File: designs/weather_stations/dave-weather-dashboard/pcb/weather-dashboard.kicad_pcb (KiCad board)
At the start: 2 copper layers, 34.5 x 58 mm, 14 parts, among them J1 Conn_01x02_MountingPin, Q1 SL2301S, SW2 SW_Omron_B3FS, U1 WEMOS_S2_Mini, U3 MCP73831-2-OT, U4 U4

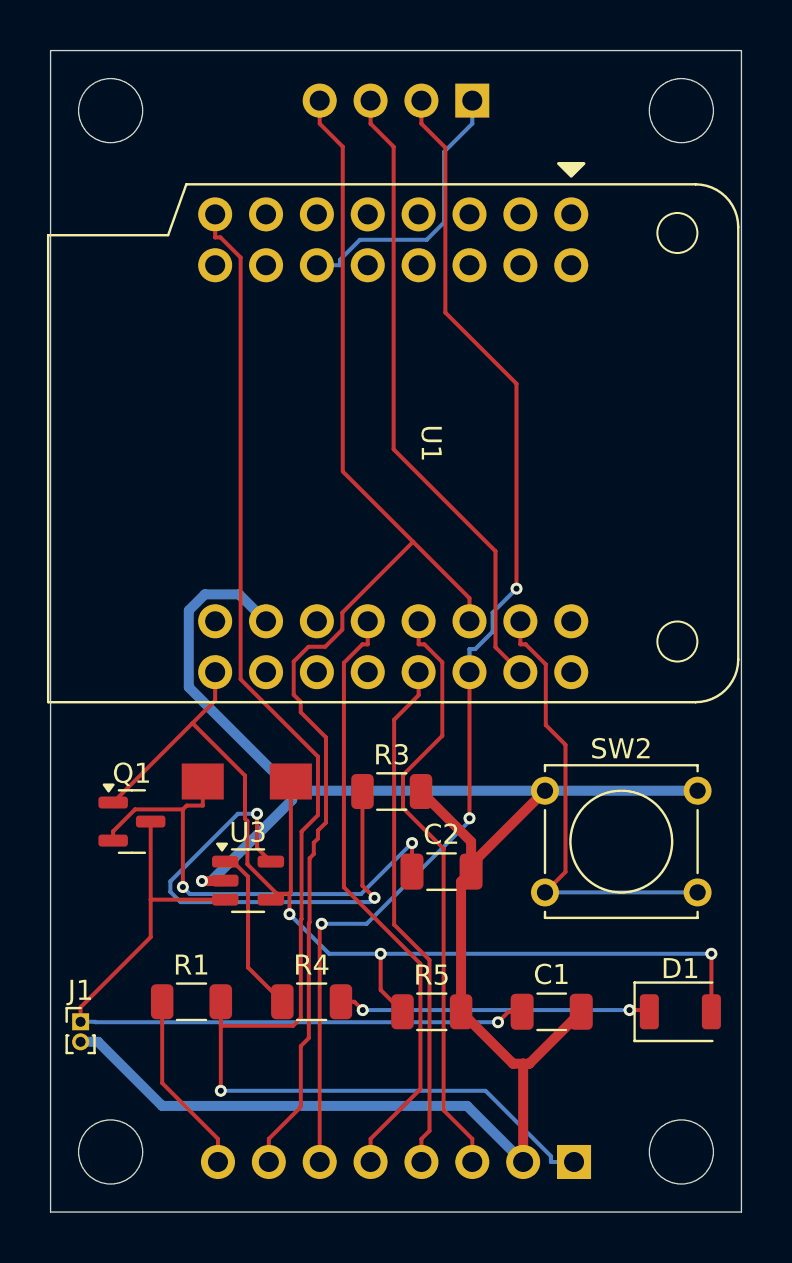
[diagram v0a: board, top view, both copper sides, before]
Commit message: done :)
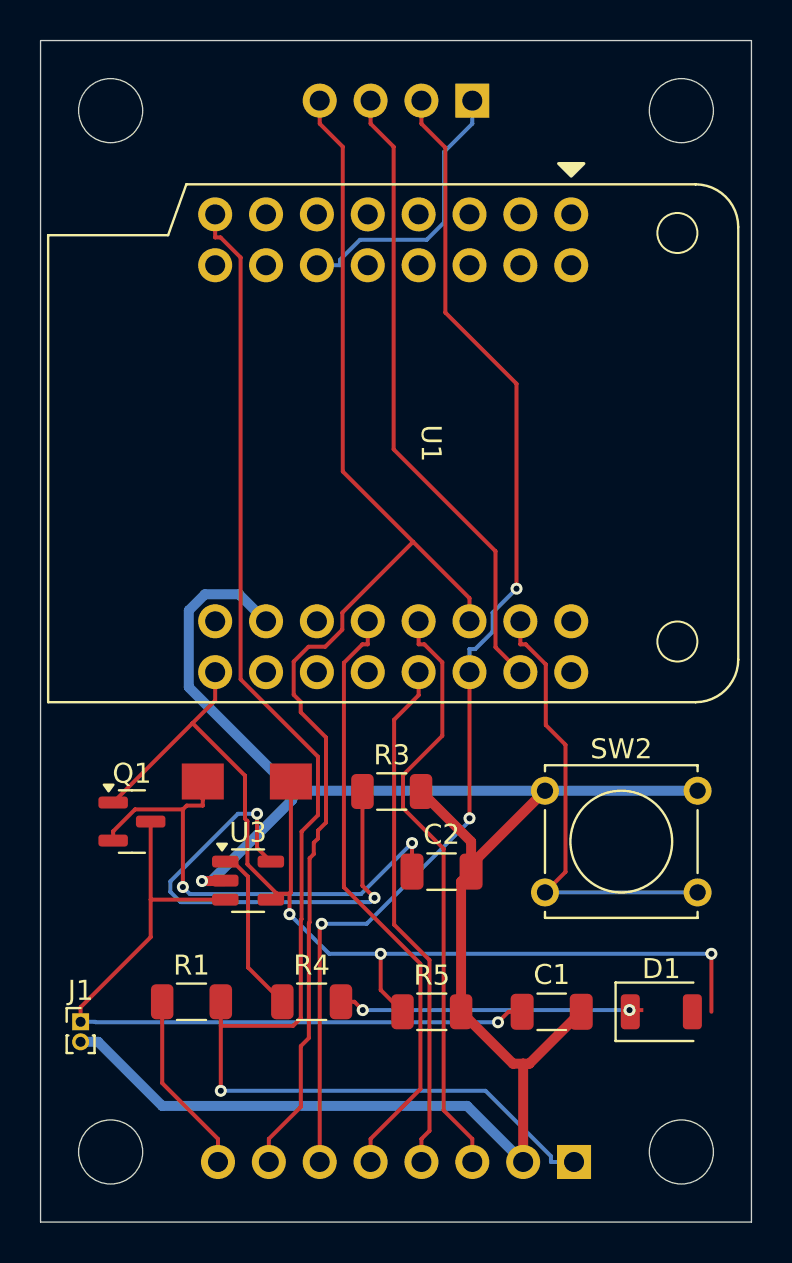
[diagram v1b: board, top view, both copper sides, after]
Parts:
- moved D1 0.95 mm to (168.0, 114.0)
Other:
- board size 34.5 x 58 mm -> 35.5 x 59 mm
